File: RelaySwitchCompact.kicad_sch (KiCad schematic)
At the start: 12 parts, among them J1 Conn_01x05_Pin, K1 1-1721150-0, U1 FOD817ASD, U2 FMMT634QTA

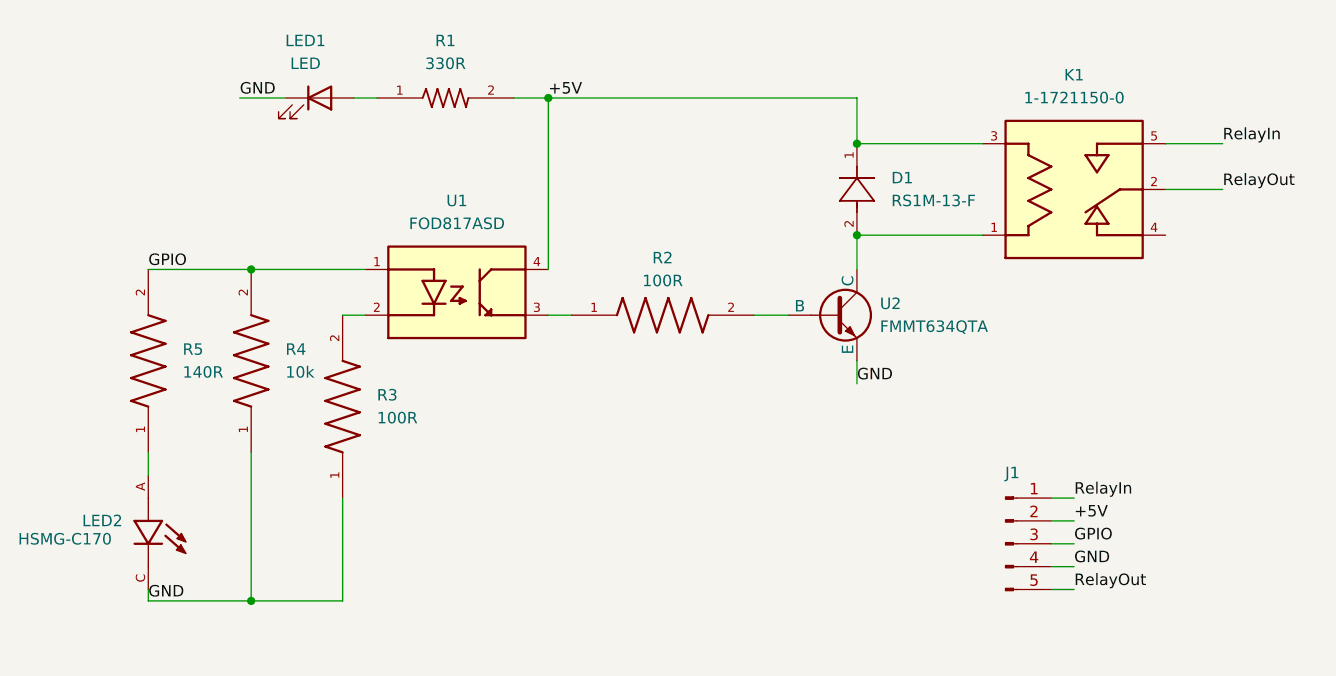
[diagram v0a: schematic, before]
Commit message: updated and cleaned up files.
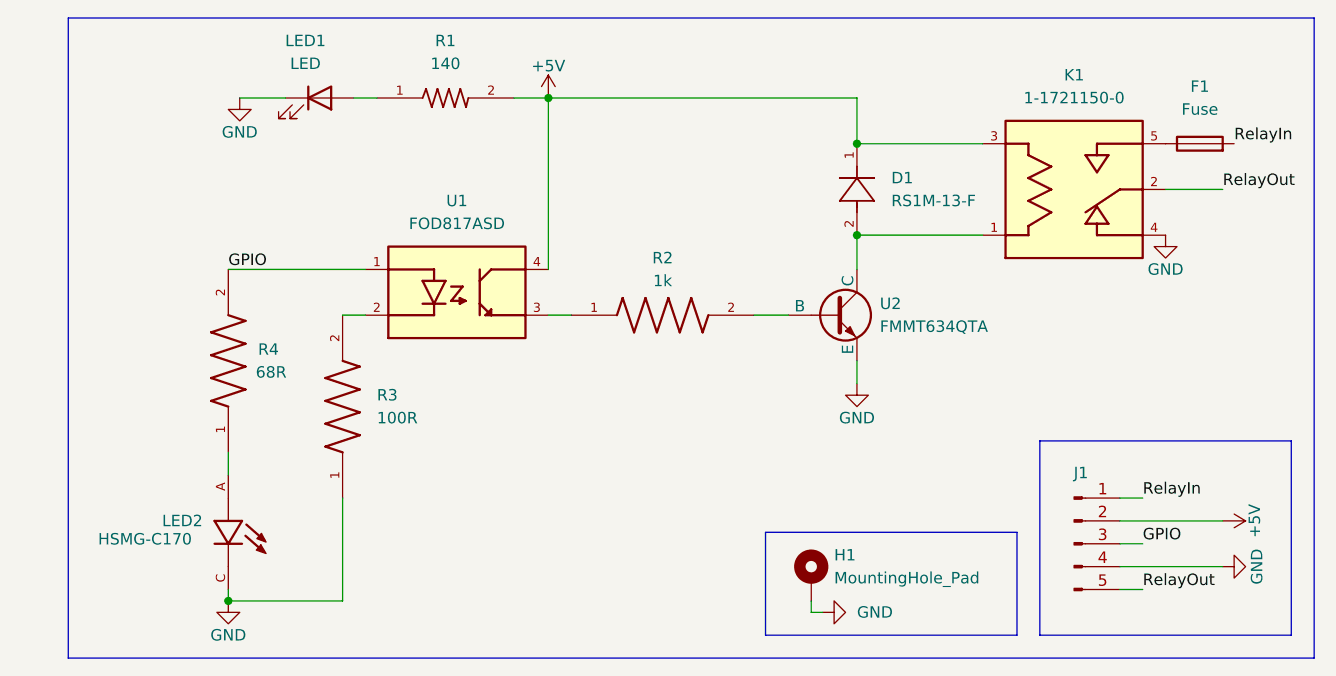
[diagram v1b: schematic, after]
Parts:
- removed R4: 10k, CRCW060310K0DHEAP:RESC1508X50N, symbol CRCW060310K0DHEAP:CRCW060310K0DHEAP
- added F1: Fuse, Diode_SMD:D_0402_1005Metric_Pad0.77x0.64mm_HandSolder, symbol Device:Fuse
- added H1: MountingHole_Pad, MountingHole:MountingHole_3.7mm_Pad, symbol Mechanical:MountingHole_Pad
- J1: value Conn_01x05_Pin -> 350-10-105-00-001101
- R1: value 330R -> 140
- R2: value 100R -> 1k; footprint AC0603JR-07100RL:RESC1608X55N -> RG1608N-102-D-T5:RESC1608X50N
- R4: renamed from R5; value 140R -> 68R
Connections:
- net GND: now also K1.4, H1.1
- net RelayIn: now also F1.2; no longer K1.5
- new net: F1.1, K1.5
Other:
- moved on the sheet: J1, LED2, R4
